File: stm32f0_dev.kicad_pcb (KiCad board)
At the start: 2 copper layers, 21.5 x 41.2 mm, 34 parts, among them J1 USB_C_Receptacle_USB2.0, J2 left_bank, J3 SWD_header, J4 right_bank, SW1 SW_Push, SW2 SW_SPDT, U1 STM32F030K6Tx, U2 AP2112K-3.3, U3 SN74LVC2G04DCKR, U4 CH340C, U5 MT29F2G01ABAGDWB, Y1 16MHz

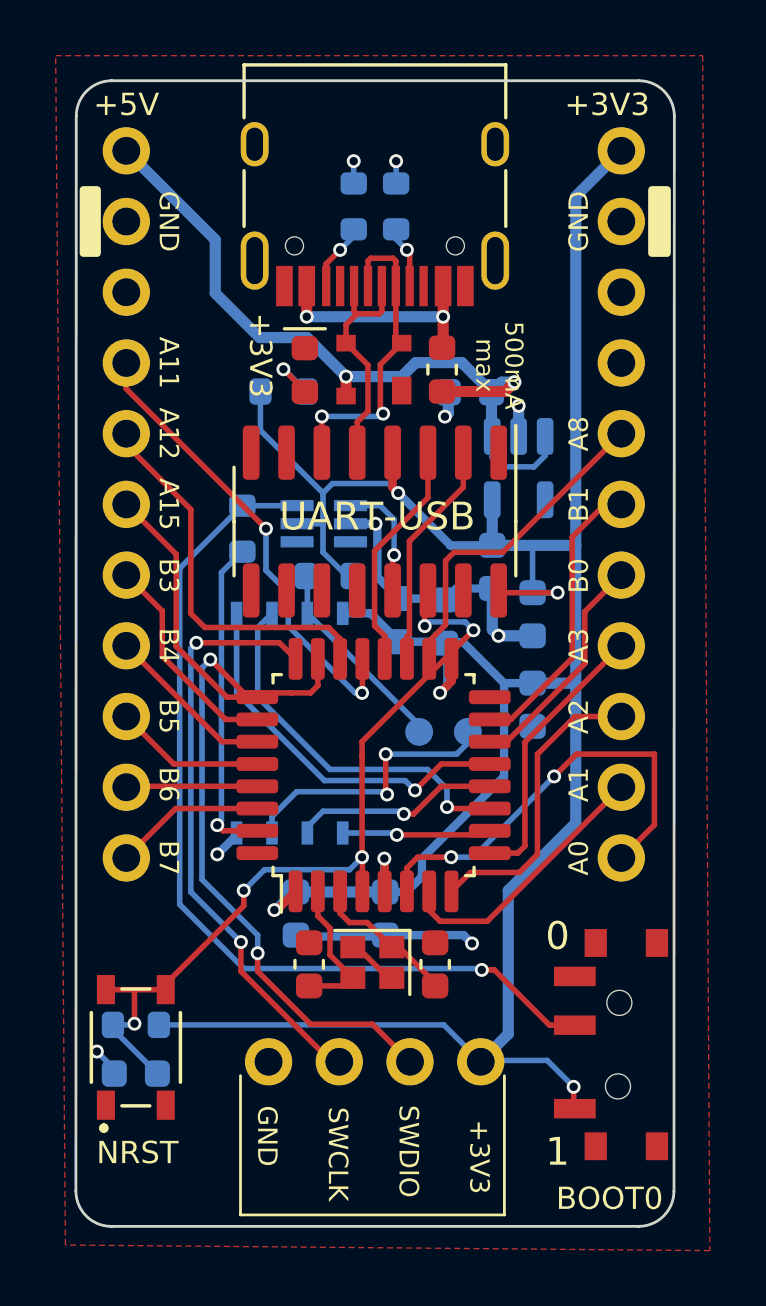
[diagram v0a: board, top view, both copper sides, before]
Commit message: Finished board, added gerber folder, uart leds, board dimensions
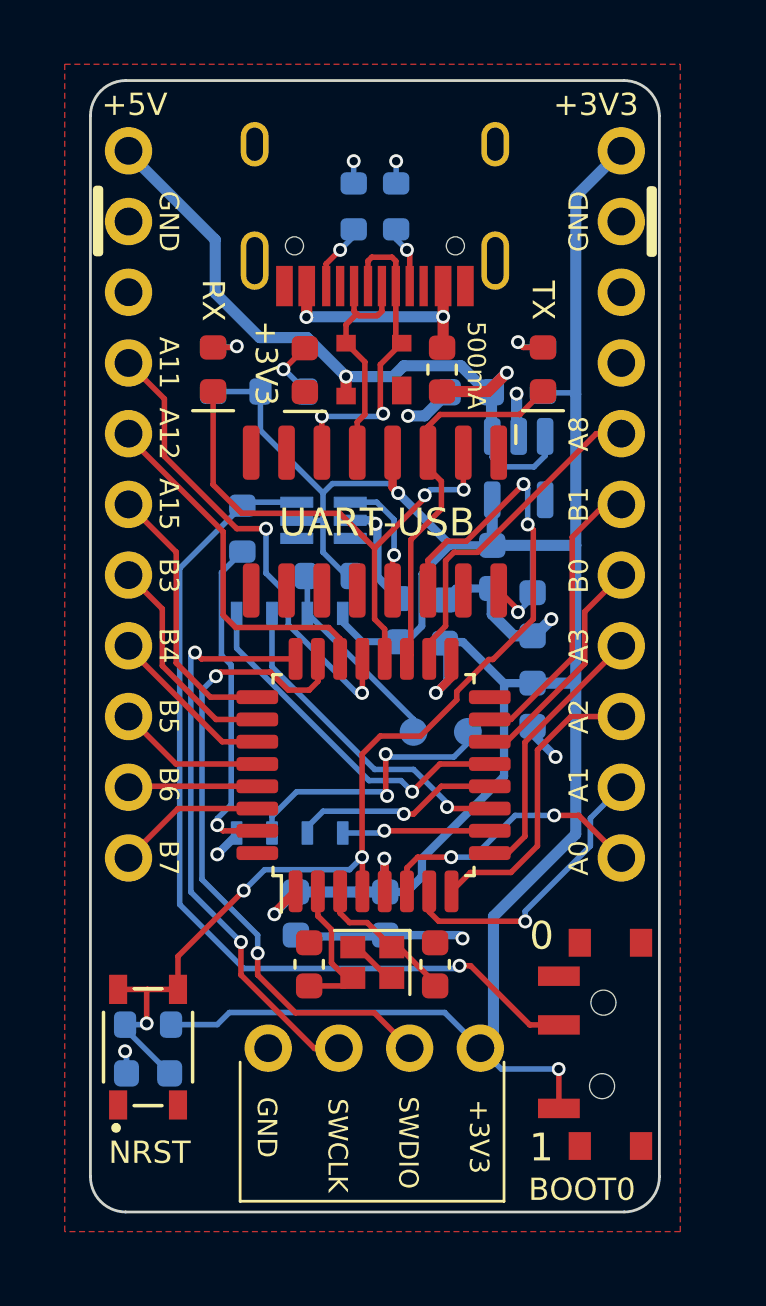
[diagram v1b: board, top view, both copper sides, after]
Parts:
- added D3: RED, LED_SMD:LED_0603_1608Metric, F.Cu at (160.5, 99.9)
- added D4: RED, LED_SMD:LED_0603_1608Metric, F.Cu at (148.7, 99.9)
- added R7: 3k3, Resistor_SMD:R_0603_1608Metric, B.Cu at (160.5, 99.9)
- added R8: 3k3, Resistor_SMD:R_0603_1608Metric, B.Cu at (148.7, 99.9)
- TP1: value TestPoint -> HOLD
- TP2: value TestPoint -> WP
- moved SW2 0.57 mm to (162.7, 124.1)
- moved J3 0.49 mm to (158.3, 124.3)
- moved C11 0.44 mm to (146.3, 125.2)
- moved R6 0.44 mm to (146.3, 123.5)
- moved SW1 0.44 mm to (146.3, 124.3)
- moved TP1 0.20 mm to (155.9, 112.9)
- moved U3 0.13 mm to (152.6, 105.3)
- moved J2 0.08 mm to (145.6, 92.1)
- turned D1 to 90 degrees
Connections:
- U4 pad 2: /TX -> /RX
- U4 pad 3: /RX -> /TX
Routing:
- net /RX: track 8.35 -> 19.7 mm, vias 0 -> 2
- net /NRST: track 30.4 -> 39.8 mm
- net /PA0: track 15.6 -> 9.96 mm
- net /TX: track 8.25 -> 13.7 mm
- net +3V3: track 108.6 -> 112.8 mm
- net Net-(D3-Pad2): track 0.00 -> 1.95 mm, vias 0 -> 1
- net Net-(D4-Pad2): track 0.00 -> 1.73 mm, vias 0 -> 1
- net /SCK: track 13.6 -> 11.9 mm
- net /PA13/SWDIO: track 24.4 -> 23.2 mm
- net GND: track 24.6 -> 25.7 mm, vias 9 -> 10
- net /MOSI: track 13.8 -> 12.9 mm
- net /PA1: track 9.74 -> 10.6 mm, vias 0 -> 1
- net /PA12: track 13.9 -> 13.2 mm
- net /PA14/SWDCLK: track 21.3 -> 20.7 mm
- net /PA11: track 16.7 -> 17.3 mm
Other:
- board size 21.5 x 41.2 mm -> 20.4 x 40.6 mm
- board text added: "500mA"
- board text added: "JLCJLCJLCJLC"
- board text added: "MT29F2G0 1ABAGDWB"
- board text added: "RX"
- board text added: "TX"
- board text removed: "500mA max"
